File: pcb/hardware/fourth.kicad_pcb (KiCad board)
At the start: 2 copper layers, 44.9 x 44.9 mm, 84 parts, among them J1 Conn_01x04, J10 Conn_01x04, J11 Conn_01x04, J12 Conn_01x06, J3 USB_B_Micro, J5 Conn_01x04, J6 Conn_01x06, J7 Conn_01x03_Pin, J8 Conn_01x03_Pin, J9 Conn_01x04, U1 BMP280, U2 MAX7456EUI_, U3 STM32F405RGTx, U4 USBLC6-2SC6, U5 ICM-20948, U6 AP63203WU, U7 LD39015M18R, U8 NTS0104PW, Y1 16Mhz, Y2 SG-210STF

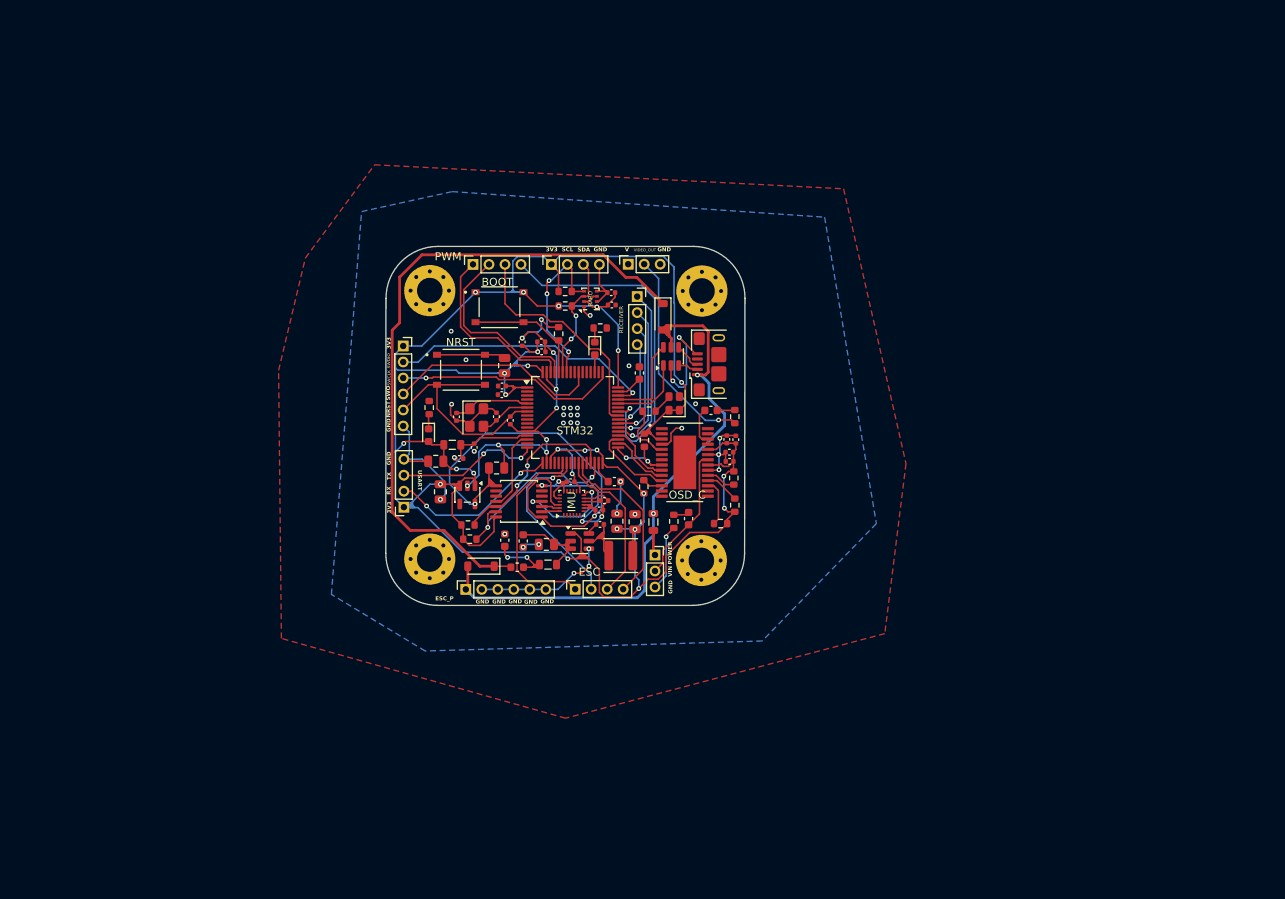
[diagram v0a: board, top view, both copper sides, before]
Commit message: Update pcb
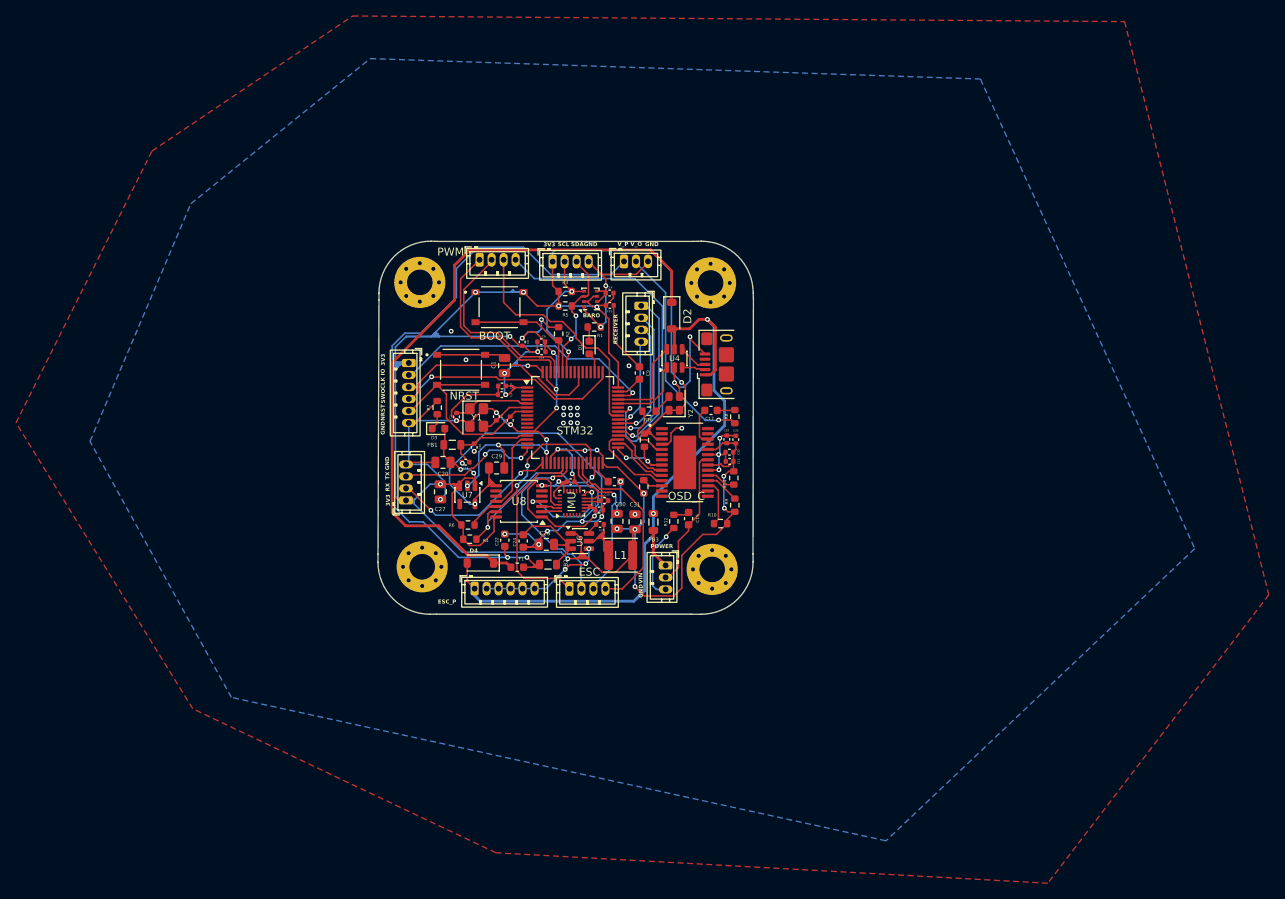
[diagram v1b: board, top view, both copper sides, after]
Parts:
- J1, J10, J11, J5, J9: footprint Connector_PinSocket_2.00mm:PinSocket_1x04_P2.00mm_Vertical -> Connector_JST:JST_ZH_B4B-ZR_1x04_P1.50mm_Vertical
- J12, J6: footprint Connector_PinSocket_2.00mm:PinSocket_1x06_P2.00mm_Vertical -> Connector_JST:JST_ZH_B6B-ZR_1x06_P1.50mm_Vertical
- J7, J8: footprint Connector_PinSocket_2.00mm:PinSocket_1x03_P2.00mm_Vertical -> Connector_JST:JST_ZH_B3B-ZR_1x03_P1.50mm_Vertical
- moved J6 2.24 mm to (108.2, 66.5), turned to -90 degrees
- moved J8 1.86 mm to (140.2, 91.8), turned to -90 degrees
- moved H4 1.75 mm to (146.1, 92.3)
- moved H1 1.62 mm to (109.5, 56.5)
- moved D3 1.49 mm to (111.9, 74.7), turned to 0 degrees
- moved H2 1.47 mm to (145.9, 56.5)
- moved H3 1.35 mm to (109.8, 92.0)
- moved J9 1.25 mm to (137.2, 59.4), turned to -90 degrees
- moved D2 1.11 mm to (141.0, 60.6)
- moved J12 1.10 mm to (116.4, 94.7), turned to 0 degrees
- moved J11 1.01 mm to (117.0, 53.6), turned to 0 degrees
- moved R7 1.00 mm to (111.7, 72.1)
- moved J3 0.95 mm to (147.8, 66.7)
- moved C20 0.92 mm to (112.4, 79.0)
- moved C18 0.90 mm to (115.2, 78.9)
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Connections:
- C22 pad 1: Net-(C22-Pad1) -> V
- F1 pad 1: Net-(C22-Pad1) -> V
- FB2 pad 1: Net-(C22-Pad1) -> V
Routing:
- net V: track 0.00 -> 84.3 mm, vias 0 -> 2
- net GND: track 185.4 -> 245.9 mm, vias 47 -> 50
- net Net-(C22-Pad1): track 9.00 -> 0.00 mm, vias 2 -> 0
- net ESC_P: track 77.7 -> 81.6 mm
- net /BUCK_IN: track 13.3 -> 15.8 mm
- net SCL: track 21.1 -> 18.7 mm, vias 3 -> 2
- net TM3_CH4: track 21.8 -> 23.9 mm
- net Net-(J8-Pin_1): track 3.15 -> 5.01 mm
- net TIM4_CH4: track 44.1 -> 45.9 mm
- net VIDEO_OUT: track 26.6 -> 27.7 mm
- net SDA: track 15.9 -> 17.0 mm
- net Net-(D2-K): track 84.1 -> 85.0 mm
- net TIM1_CH1: track 23.2 -> 24.0 mm
- net TIM4_CH3: track 28.8 -> 29.6 mm
- net USB_CONN_D-: track 2.55 -> 3.33 mm
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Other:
- board size 44.9 x 44.9 mm -> 46.9 x 46.6 mm
- board text added: "C2"
- board text added: "CLK"
- board text added: "IO"
- board text added: "V_O"
- board text added: "V_P"
- board text added: "https://github.com/Bhakti-A/Maya_V_FlightController/"
- board text removed: "SWCLK"
- board text removed: "SWDIO"
- board text removed: "USART"
- board text removed: "V"
- board text removed: "VIDEO_OUT"
